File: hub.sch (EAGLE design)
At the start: 27 parts, among them U1 10118194-MICRO-USB, U2 LM3671MF-3.3/NOPBMF05A-M, U3 SN74LVC1T45DBVRDBV6-M, U4 SN74LVC1T45DBVRDBV6-M

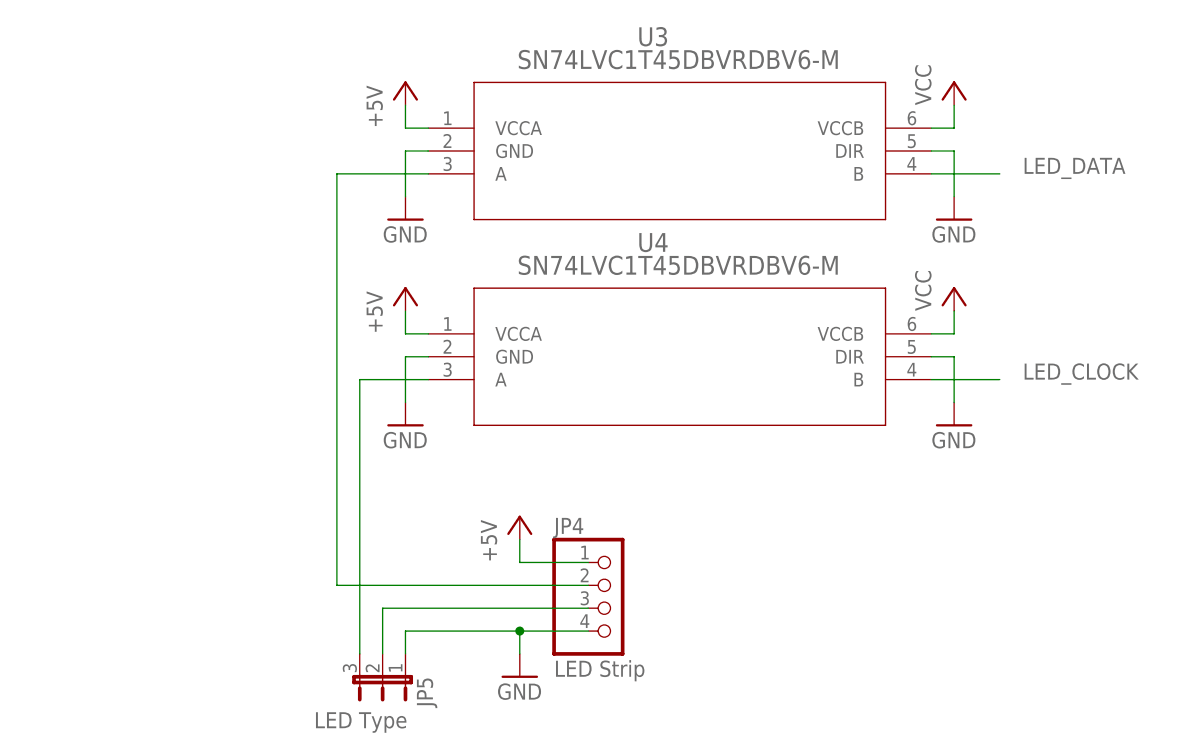
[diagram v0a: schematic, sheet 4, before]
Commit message: Tweaked and confirmed some connections
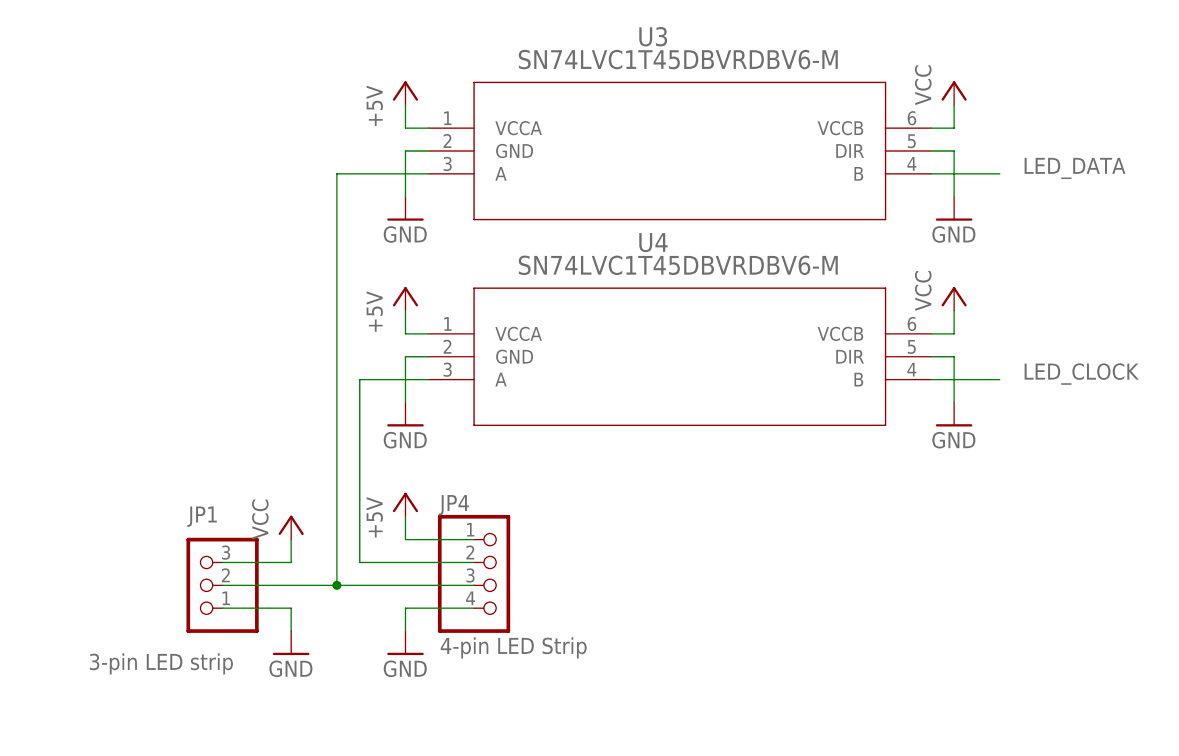
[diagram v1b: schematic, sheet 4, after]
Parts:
- removed JP5: LED Type, jumper:JP2E
- removed JP6: JTAG Enable, jumper:JP2E
- added JP3: JTAG, pinhead:PINHD-2X3
- JP1: value JTAG -> 3-pin LED strip; device pinhead:PINHD-1X6 -> pinhead:PINHD-1X3/90
- JP4: value LED Strip -> 4-pin LED Strip
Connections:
- removed net N$7: JP4.3, JP5.2
- removed net TRST_N: JP1.1, JP6.1
- net EN: now also JP3.1; no longer JP6.2, JP6.3
- net GND: now also JP1.1, JP3.6; no longer JP1.6, JP5.1
- net N$8: now also JP1.2, JP4.3; no longer JP4.2
- net N$9: now also JP4.2; no longer JP5.3
- net TCK: now also JP3.4; no longer JP1.4
- net TDI: now also JP3.3; no longer JP1.3
- net TDO: now also JP3.2; no longer JP1.2
- net TMS: now also JP3.5; no longer JP1.5
- net VCC: now also JP1.3
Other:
- moved on the sheet: JP4
